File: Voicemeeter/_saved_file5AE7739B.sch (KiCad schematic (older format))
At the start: 16 parts

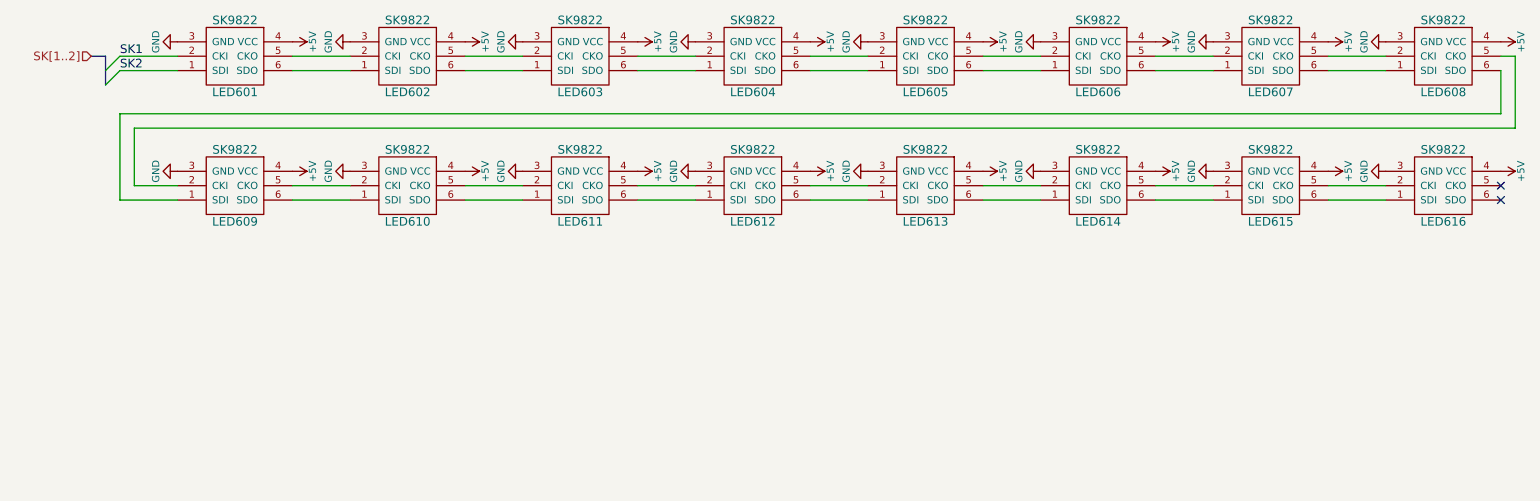
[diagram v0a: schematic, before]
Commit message: fsd
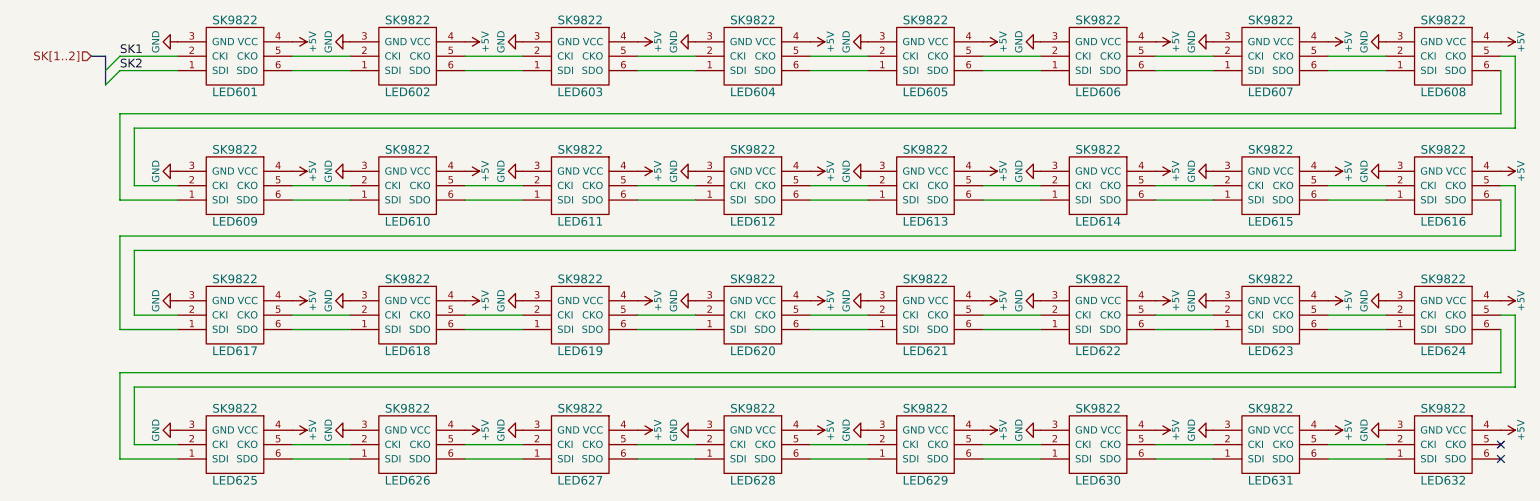
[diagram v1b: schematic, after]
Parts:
- added LED617, LED618, LED619, LED620, LED621, LED622, LED623, LED624, LED625, LED626, LED627, LED628, LED629, LED630, LED631, LED632: SK9822, LEDs:LED_RGB_5050-6, symbol SK9822
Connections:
- net +5V: now also LED617.4 (VCC), LED618.4 (VCC), LED619.4 (VCC), LED620.4 (VCC), LED621.4 (VCC), LED622.4 (VCC), LED623.4 (VCC), LED624.4 (VCC), LED625.4 (VCC), LED626.4 (VCC), LED627.4 (VCC), LED628.4 (VCC), LED629.4 (VCC), LED630.4 (VCC), LED631.4 (VCC), LED632.4 (VCC)
- net GND: now also LED617.3 (GND), LED618.3 (GND), LED619.3 (GND), LED620.3 (GND), LED621.3 (GND), LED622.3 (GND), LED623.3 (GND), LED624.3 (GND), LED625.3 (GND), LED626.3 (GND), LED627.3 (GND), LED628.3 (GND), LED629.3 (GND), LED630.3 (GND), LED631.3 (GND), LED632.3 (GND)
- net at LED616.5 (CKO): now also LED617.2 (CKI)
- net at LED616.6 (SDO): now also LED617.1 (SDI)
- new net: LED617.5 (CKO), LED618.2 (CKI)
- new net: LED617.6 (SDO), LED618.1 (SDI)
- new net: LED618.5 (CKO), LED619.2 (CKI)
- new net: LED618.6 (SDO), LED619.1 (SDI)
- new net: LED619.5 (CKO), LED620.2 (CKI)
- new net: LED619.6 (SDO), LED620.1 (SDI)
- new net: LED620.5 (CKO), LED621.2 (CKI)
- new net: LED620.6 (SDO), LED621.1 (SDI)
- new net: LED621.5 (CKO), LED622.2 (CKI)
- new net: LED621.6 (SDO), LED622.1 (SDI)
- new net: LED622.5 (CKO), LED623.2 (CKI)
- new net: LED622.6 (SDO), LED623.1 (SDI)
- new net: LED623.5 (CKO), LED624.2 (CKI)
- new net: LED623.6 (SDO), LED624.1 (SDI)
- new net: LED624.5 (CKO), LED625.2 (CKI)
- new net: LED624.6 (SDO), LED625.1 (SDI)
- new net: LED625.5 (CKO), LED626.2 (CKI)
- new net: LED625.6 (SDO), LED626.1 (SDI)
- new net: LED626.5 (CKO), LED627.2 (CKI)
- new net: LED626.6 (SDO), LED627.1 (SDI)
- new net: LED627.5 (CKO), LED628.2 (CKI)
- new net: LED627.6 (SDO), LED628.1 (SDI)
- new net: LED628.5 (CKO), LED629.2 (CKI)
- new net: LED628.6 (SDO), LED629.1 (SDI)
- new net: LED629.5 (CKO), LED630.2 (CKI)
- new net: LED629.6 (SDO), LED630.1 (SDI)
- new net: LED630.5 (CKO), LED631.2 (CKI)
- new net: LED630.6 (SDO), LED631.1 (SDI)
- new net: LED631.5 (CKO), LED632.2 (CKI)
- new net: LED631.6 (SDO), LED632.1 (SDI)
